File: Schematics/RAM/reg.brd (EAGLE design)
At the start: 42 x 47.9 mm, 19 parts

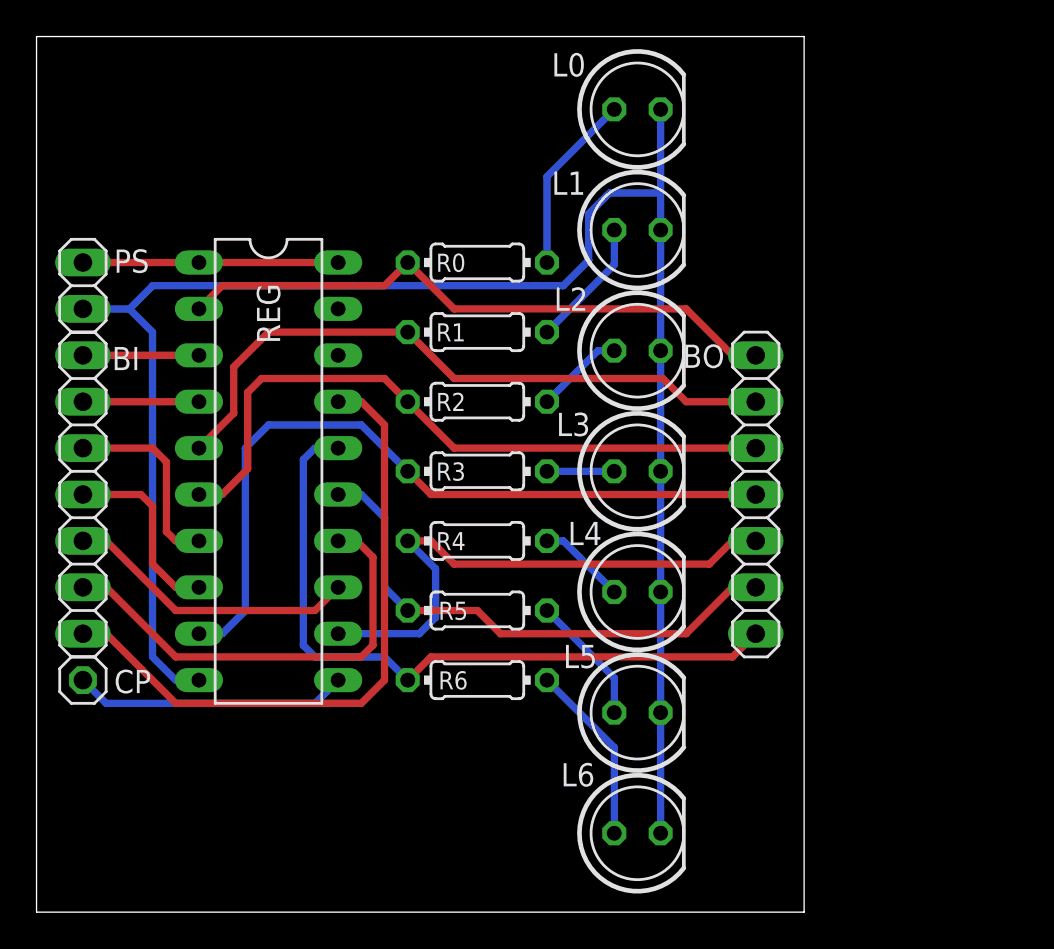
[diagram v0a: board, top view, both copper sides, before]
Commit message: Fixed major mistakes.
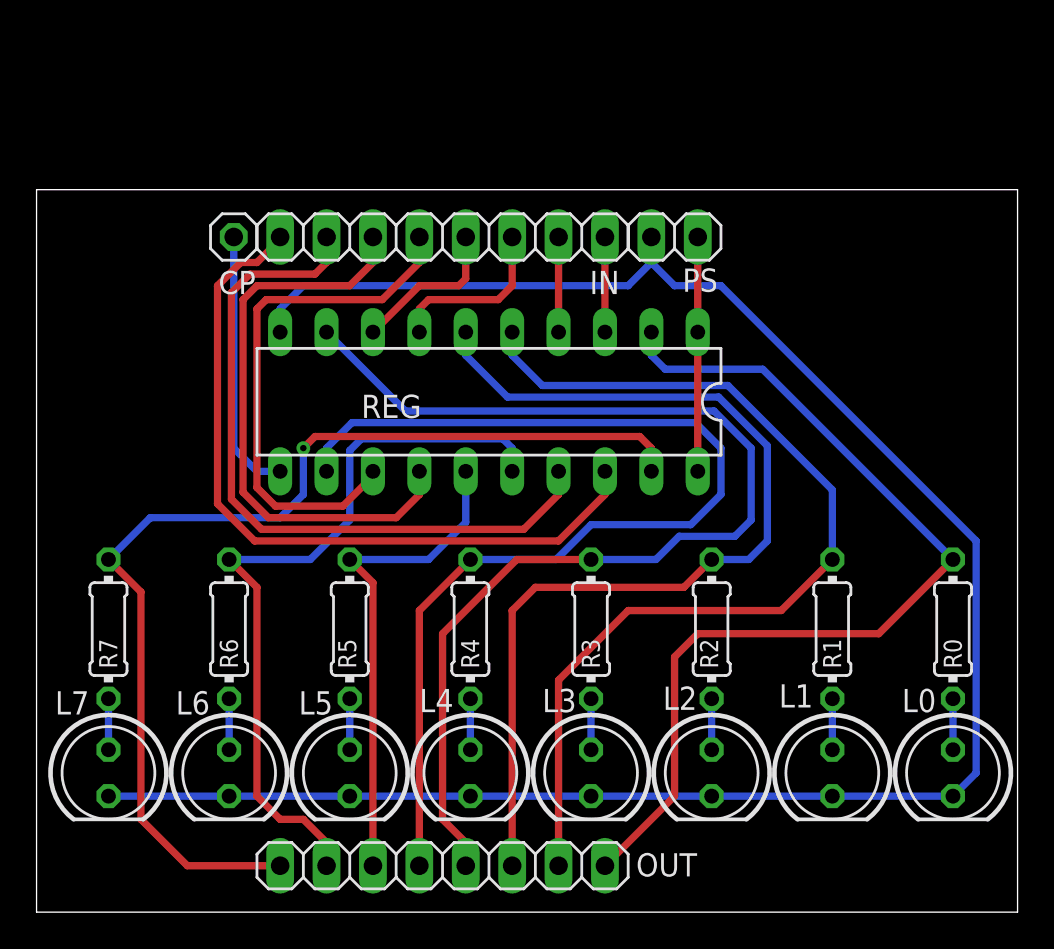
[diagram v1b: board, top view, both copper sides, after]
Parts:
- removed BI, BO: (no value), pinhead:1X07
- added IN, OUT: (no value), pinhead:1X08
- added L7: (no value), led:LED5MM
- added R7: (no value), rcl:0204/7
- moved L0 40.2 mm to (50.2, 7.62), turned to 270 degrees
- moved R0 32.9 mm to (50.2, 15.5), turned to 90 degrees
- moved PS 32.5 mm to (34.9, 37.0), turned to 0 degrees
- moved L1 31.6 mm to (43.6, 7.62), turned to 270 degrees
- moved CP 25.6 mm to (10.8, 37.0)
- moved R1 25.3 mm to (43.6, 15.5), turned to 90 degrees
- moved L2 23.5 mm to (37.0, 7.62), turned to 270 degrees
- moved L6 22.6 mm to (10.5, 7.62), turned to 270 degrees
- moved R2 17.9 mm to (37.0, 15.5), turned to 90 degrees
- moved L3 16.7 mm to (30.4, 7.62), turned to 270 degrees
- moved L5 16.1 mm to (17.1, 7.62), turned to 270 degrees
- moved R6 13.9 mm to (10.5, 15.5), turned to 90 degrees
- moved L4 13.5 mm to (23.7, 7.62), turned to 270 degrees
- moved REG 12.7 mm to (24.8, 27.9), turned to 180 degrees
- moved R3 10.6 mm to (30.4, 15.5), turned to 90 degrees
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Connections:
- new net B7: IN.1, REG.18
- new net N$8: L7.A, R7.1
- new net O7: OUT.1, R7.2, REG.19
- net B0: now also IN.8; no longer BI.7
- net B1: now also IN.7; no longer BI.6
- net B2: now also IN.6; no longer BI.5
- net B3: now also IN.5; no longer BI.4
- net B4: now also IN.4; no longer BI.3
- net B5: now also IN.3; no longer BI.2
- net B6: now also IN.2; no longer BI.1
- net GND: now also L7.K
- net O0: now also OUT.8; no longer BO.7
- net O1: now also OUT.7; no longer BO.6
- net O2: now also OUT.6; no longer BO.5
- net O3: now also OUT.5; no longer BO.4
- net O4: now also OUT.4; no longer BO.3
- net O5: now also OUT.3; no longer BO.2
- net O6: now also OUT.2; no longer BO.1
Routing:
- net O7: track 0.00 -> 59.2 mm, vias 0 -> 1
- net B7: track 0.00 -> 40.9 mm
- net O4: track 30.6 -> 59.7 mm
- net O3: track 42.0 -> 62.5 mm
- net O0: track 33.6 -> 52.9 mm
- net O2: track 37.1 -> 54.6 mm
- net O1: track 36.2 -> 53.5 mm
- net B4: track 16.1 -> 28.8 mm
- net GND: track 98.0 -> 108.9 mm
- net N$7: track 9.91 -> 2.79 mm
- net N$1: track 9.91 -> 2.79 mm
- net B5: track 24.8 -> 31.9 mm
- net N$2: track 7.11 -> 2.79 mm
- net N$6: track 7.11 -> 2.79 mm
- net B6: track 35.7 -> 39.2 mm
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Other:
- board size 42 x 47.9 mm -> 53.7 x 39.5 mm
